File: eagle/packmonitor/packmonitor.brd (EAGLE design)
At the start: 100 x 18 mm, 12 parts, among them IC2 24C64

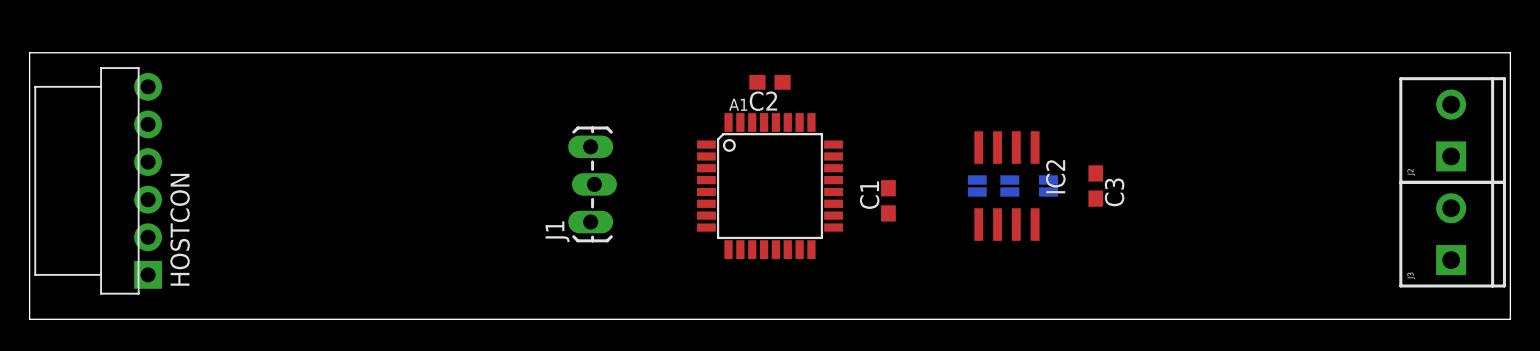
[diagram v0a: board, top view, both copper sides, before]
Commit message: making good progress on schematic and board layout
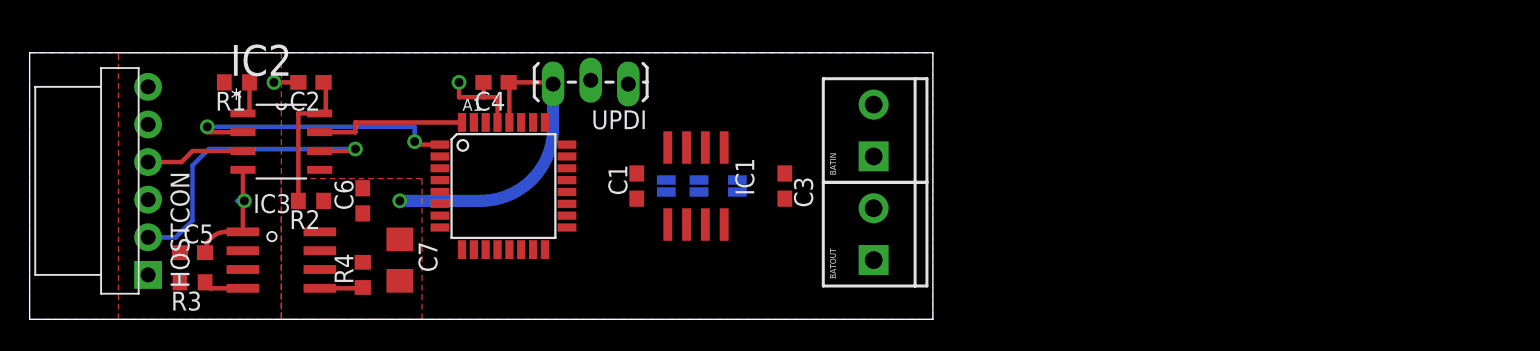
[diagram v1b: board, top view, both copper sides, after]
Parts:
- removed J1: (no value), SparkFun-Connectors:1X03_LOCK_LONGPADS
- removed J2, J3: (no value), SparkFun-Connectors:SCREWTERMINAL-3.5MM-2
- added BATIN, BATOUT: (no value), SparkFun-Connectors:SCREWTERMINAL-3.5MM-2
- added C4, C5, C6: 100n, rcl:C0603
- added C7: 120u, rcl:C1206
- added IC1: 24C64, microchip:SO-08
- added IC3: AP2411, ti-special:SO08
- added R1, R3, R4: 10K, rcl:R0603
- added R2: (no value), rcl:R0603
- added UPDI: (no value), SparkFun-Connectors:1X03_LOCK_LONGPADS
- A1: value ATMEGA4808-TQFN32A -> ATMEGA4808
- C1, C2, C3: value 100u -> 100n
- IC2: value 24C64 -> TCA4311A; device microchip:SO-08 -> NXP_By_element14_Batch_1:SOIC127P600X175-8N
- moved IC2 49.1 mm to (17.0, 12.0), turned to 0 degrees
- moved C2 31.0 mm to (19.0, 16.0)
- moved C3 21.0 mm to (51.0, 9.00)
- moved JP1 21.0 mm to (47.8, 9.00)
- moved JP2 21.0 mm to (45.2, 9.00)
- moved JP3 21.0 mm to (43.0, 9.00)
- moved A1 18.0 mm to (32.0, 9.00)
- moved C1 17.0 mm to (41.0, 9.00)
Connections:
- removed net N$2: A1.27, J1.2
- new net BUSREADY: IC2.5, R2.1
- new net ENBUSPWR: IC3.4, R3.1
- new net N$3: HOSTCON.2, IC2.6
- new net N$4: HOSTCON.4, IC2.3
- new net N$6: IC2.1, R1.1
- new net PWRFAULT: IC3.5, R4.1
- new net UPDI: A1.27, UPDI.2
- new net VCCIO: C5.1, HOSTCON.6, IC3.2, IC3.3, R1.2, R3.2
- net A0: now also IC1.1; no longer IC2.1
- net A1: now also IC1.2; no longer IC2.2
- net A2: now also IC1.3; no longer IC2.3
- net GND: now also BATIN.2, BATOUT.1, C4.2, C5.2, C6.2, C7.2, IC1.4, IC1.7, IC3.1, UPDI.1; no longer IC2.7, J1.1
- net SCL: now also IC1.6, IC2.2; no longer HOSTCON.2, IC2.6
- net SDA: now also IC1.5, IC2.7; no longer HOSTCON.4, IC2.5
- net VCC: now also C4.1, C6.1, C7.1, IC1.8, IC3.6, IC3.7, IC3.8, R2.2, R4.2, UPDI.3; no longer HOSTCON.6, J1.3
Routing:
- net VCC: track 0.00 -> 31.2 mm, vias 0 -> 1
- net N$3: track 0.00 -> 21.2 mm, vias 0 -> 1
- net SCL: track 0.00 -> 19.7 mm, vias 0 -> 2
- net GND: track 0.00 -> 16.0 mm, vias 0 -> 3
- net SDA: track 0.00 -> 10.3 mm
- net N$4: track 0.00 -> 6.72 mm
- net PWRFAULT: track 0.00 -> 2.92 mm
- net ENBUSPWR: track 0.00 -> 2.72 mm
- net N$6: track 0.00 -> 2.54 mm
- added copper zone on layer 16, net GND
- added copper zone on layer 1, net VCC
- added copper zone on layer 1, net VCCIO
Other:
- board size 100 x 18 mm -> 61 x 18 mm
